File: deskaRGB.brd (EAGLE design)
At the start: 60.6 x 64.1 mm, 15 parts, among them T1 TIP122, T2 TIP122, T3 TIP122

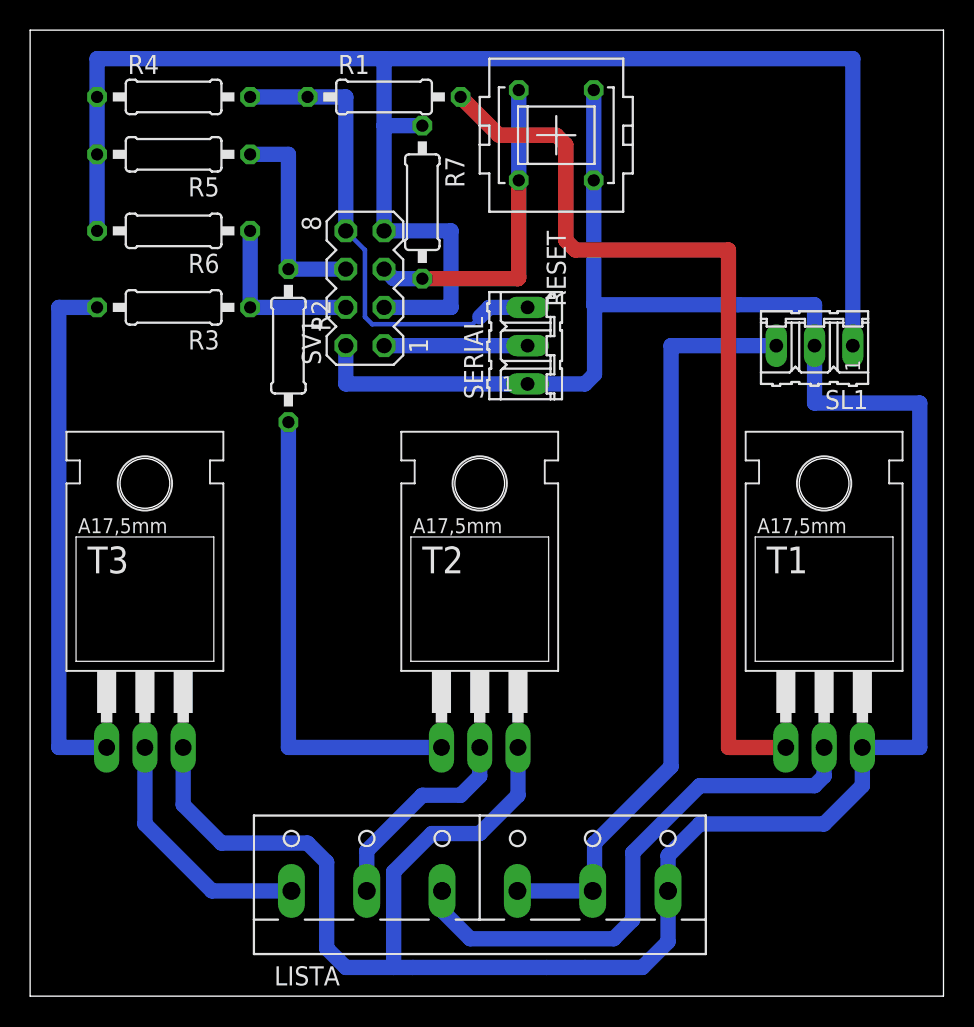
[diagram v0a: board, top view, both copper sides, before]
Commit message: +
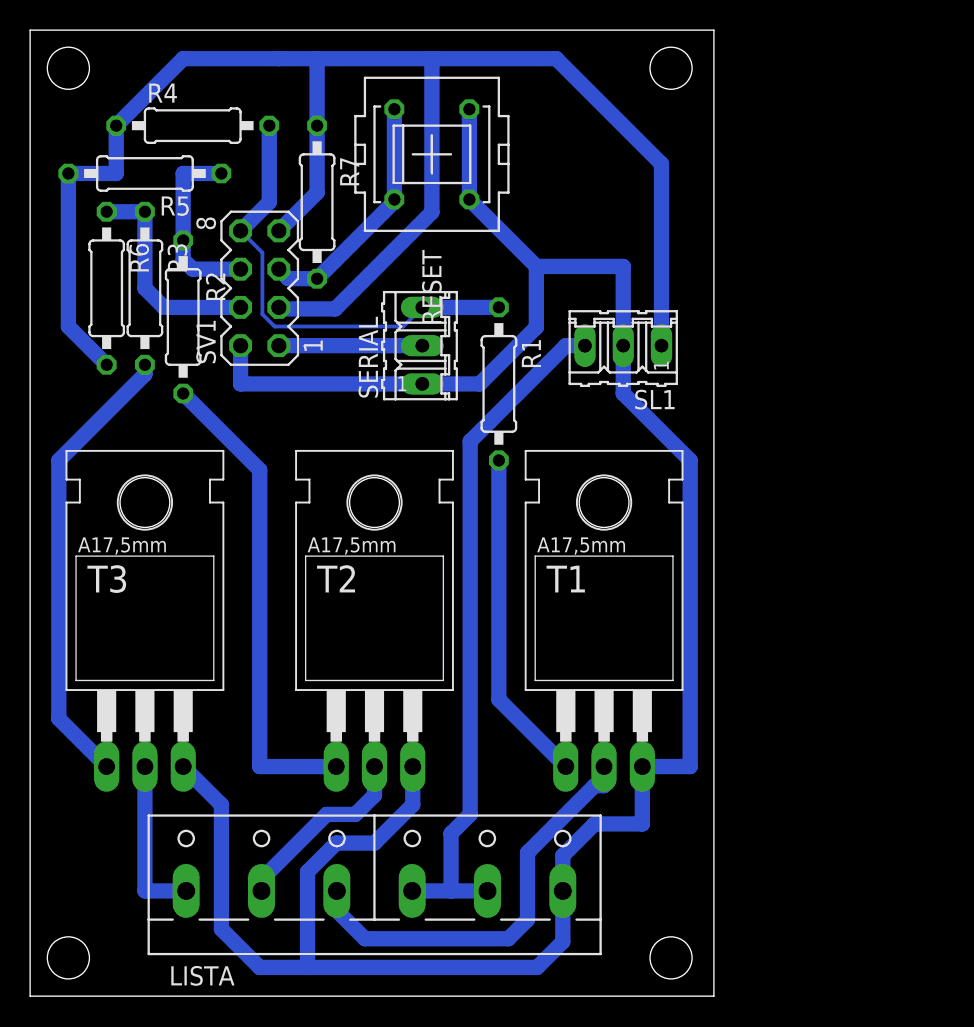
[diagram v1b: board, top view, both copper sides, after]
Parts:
- moved R1 20.5 mm to (31.1, 40.6), turned to 270 degrees
- moved T1 14.7 mm to (38.1, 21.6)
- moved SL1 12.7 mm to (39.4, 43.2)
- moved RESET 8.35 mm to (26.7, 55.9)
- moved R2 7.24 mm to (10.2, 45.1)
- moved T2 7.10 mm to (22.9, 21.6)
- moved SERIAL 6.99 mm to (26.0, 43.2)
- moved SV1 6.99 mm to (15.2, 47.0)
- moved LISTA 6.98 mm to (22.9, 8.26)
- moved R7 6.98 mm to (19.1, 52.7)
- moved R6 5.85 mm to (5.08, 47.0), turned to 270 degrees
- moved R3 2.29 mm to (7.62, 47.0), turned to 270 degrees
- moved R5 2.29 mm to (7.62, 54.6)
- moved R4 2.29 mm to (10.8, 57.8)
- moved T3 1.27 mm to (7.62, 21.6)
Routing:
- net N$4: track 62.5 -> 22.2 mm
- net GND: track 180.6 -> 153.7 mm
- net N$1: track 36.4 -> 27.9 mm
- net N$3: track 16.6 -> 11.0 mm
- net RST: track 21.7 -> 16.2 mm
- net +12V: track 50.3 -> 45.6 mm
- net N$6: track 34.9 -> 30.4 mm
- net GPIO2: track 11.4 -> 14.5 mm
- net RX: track 32.9 -> 30.5 mm
- net GPIO0: track 14.0 -> 12.3 mm
- net N$2: track 14.1 -> 12.5 mm
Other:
- board size 60.6 x 64.1 mm -> 45.4 x 64.1 mm
